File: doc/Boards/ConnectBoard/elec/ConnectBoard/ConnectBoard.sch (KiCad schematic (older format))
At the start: 20 parts

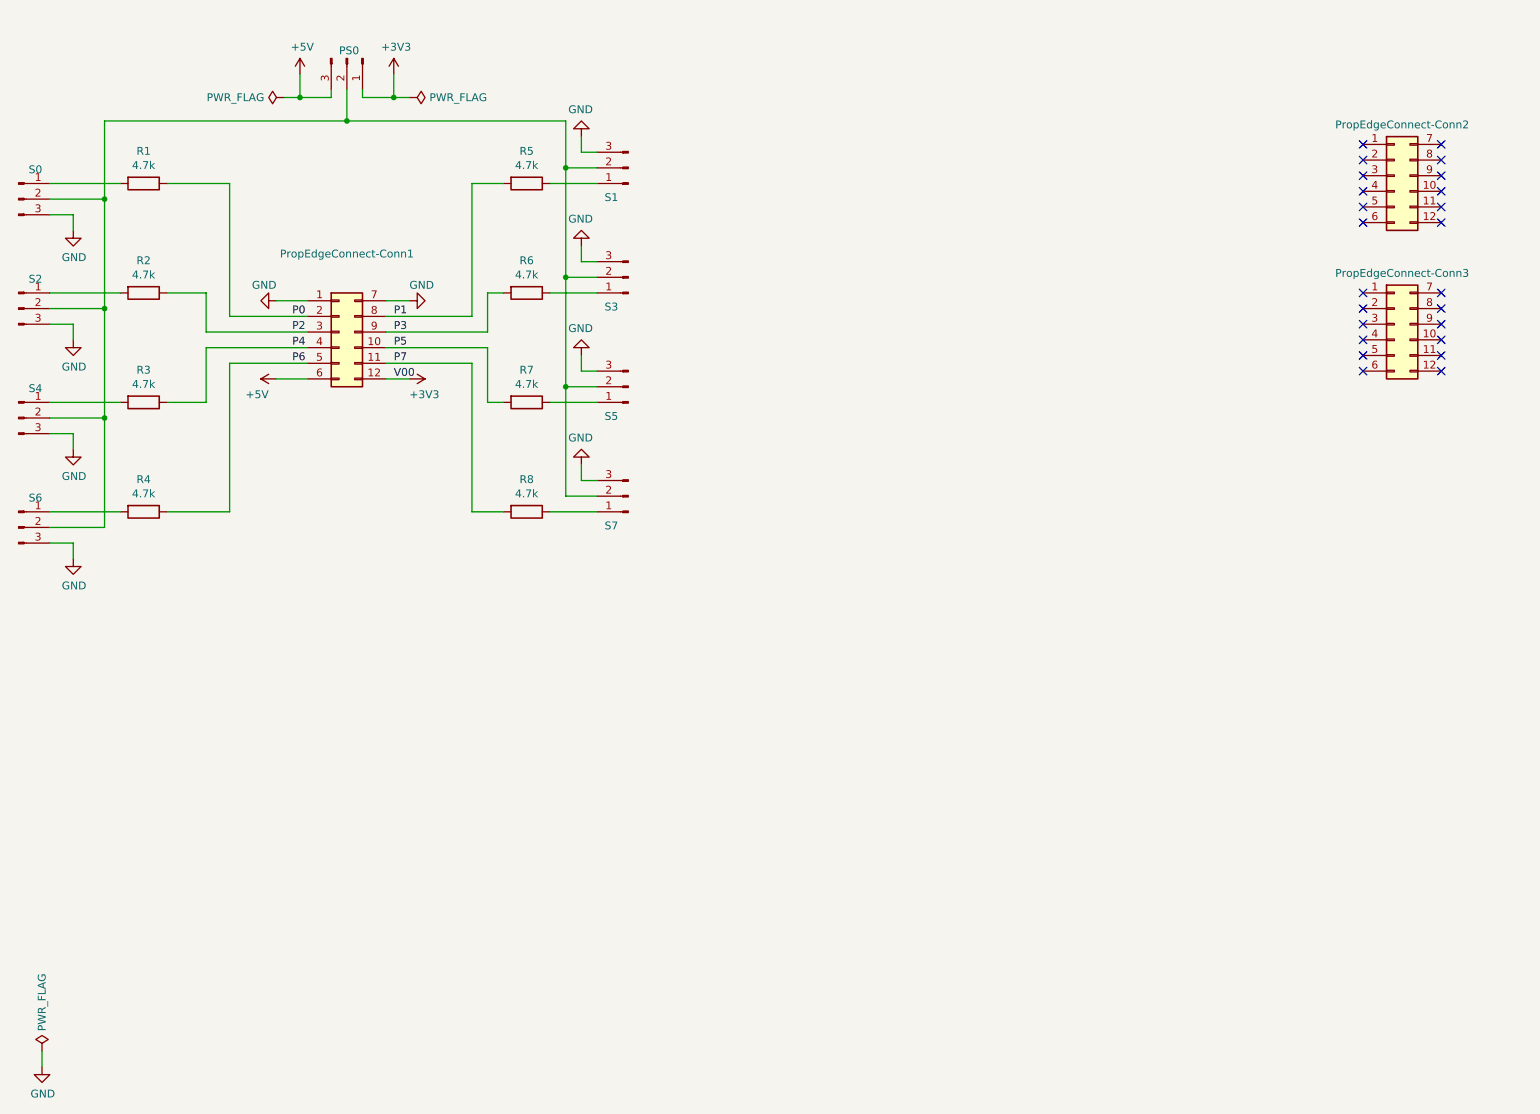
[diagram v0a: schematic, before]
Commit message: Updates
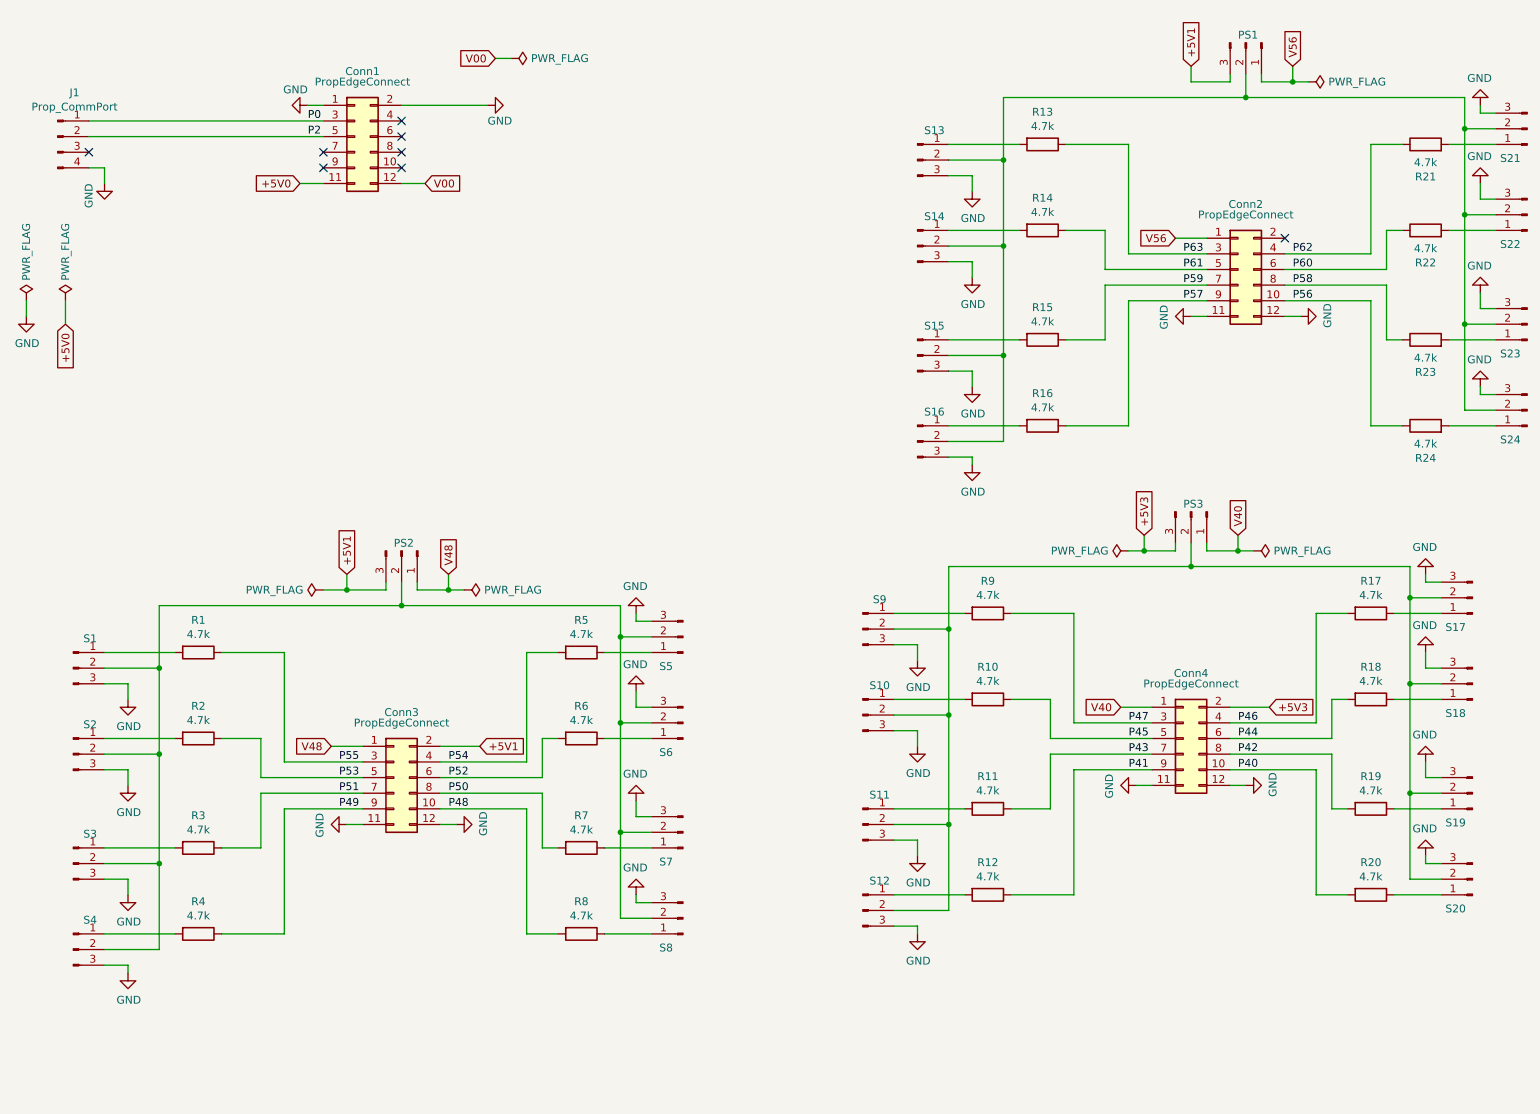
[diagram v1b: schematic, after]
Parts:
- removed PropEdgeConnect-Conn1: PropEdgeConnect-Conn1, Connector_PinSocket_2.54mm:PinSocket_2x06_P2.54mm_Vertical, symbol Connector_Generic:Conn_02x06_Top_Bottom
- removed PropEdgeConnect-Conn2: PropEdgeConnect-Conn2, Connector_PinSocket_2.54mm:PinSocket_2x06_P2.54mm_Vertical, symbol Connector_Generic:Conn_02x06_Top_Bottom
- removed PropEdgeConnect-Conn3: PropEdgeConnect-Conn3, Connector_PinSocket_2.54mm:PinSocket_2x06_P2.54mm_Vertical, symbol Connector_Generic:Conn_02x06_Top_Bottom
- added Conn1, Conn2, Conn3, Conn4: PropEdgeConnect, Connector_PinSocket_2.54mm:PinSocket_2x06_P2.54mm_Vertical, symbol Connector_Generic:Conn_02x06_Odd_Even
- added J1: Prop_CommPort, Connector_PinSocket_2.54mm:PinSocket_1x04_P2.54mm_Vertical, symbol Connector:Conn_01x04_Male
- added PS2, PS3: PowerSelect, Connector_PinHeader_2.54mm:PinHeader_1x03_P2.54mm_Vertical, symbol Connector:Conn_01x03_Male
- added R1, R10, R11, R12, R17, R18, R19, R2, R20, R3, R4, R5, R6, R7, R8, R9: 4.7k, Resistor_THT:R_Axial_DIN0207_L6.3mm_D2.5mm_P7.62mm_Horizontal, symbol Device:R
- added S1, S10, S11, S12, S17, S18, S19, S2, S20, S3, S4, S5, S6, S7, S8, S9: SonarConnect, Connector_PinHeader_2.54mm:PinHeader_1x03_P2.54mm_Vertical, symbol Connector:Conn_01x03_Male
- renumbered PS0 to PS1, R1 to R13, R2 to R14, R3 to R15, R4 to R16, R5 to R21, R6 to R22, R7 to R23, R8 to R24, S0 to S13, S2 to S14, S4 to S15, S6 to S16, S1 to S21, S3 to S22, S5 to S23, S7 to S24
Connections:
- net P1 is gone; now on an unnamed net: R21.2
- net P3 is gone; now on an unnamed net: R22.2
- net P5 is gone; now on an unnamed net: R23.2
- net P7 is gone; now on an unnamed net: R24.2
- net GND: now also Conn1.1 (Pin_1), Conn1.2 (Pin_2), Conn2.11 (Pin_11), Conn2.12 (Pin_12), Conn3.11 (Pin_11), Conn3.12 (Pin_12), Conn4.11 (Pin_11), Conn4.12 (Pin_12), J1.4 (Pin_4), S1.3 (Pin_3), S10.3 (Pin_3), S11.3 (Pin_3), S12.3 (Pin_3), S17.3 (Pin_3), S18.3 (Pin_3), S19.3 (Pin_3), S2.3 (Pin_3), S20.3 (Pin_3), S3.3 (Pin_3), S4.3 (Pin_3), S5.3 (Pin_3), S6.3 (Pin_3), S7.3 (Pin_3), S8.3 (Pin_3), S9.3 (Pin_3)
- net P0: now also Conn1.3 (Pin_3), J1.1 (Pin_1); no longer R13.1
- net P2: now also Conn1.5 (Pin_5), J1.2 (Pin_2); no longer R14.1
- net at S21.1 (Pin_1): no longer R21.1
- net at S22.1 (Pin_1): no longer R22.1
- net at S23.1 (Pin_1): no longer R23.1
- net at S24.1 (Pin_1): no longer R24.1
- net +3V3 renamed V56
- net V56: now also Conn2.1 (Pin_1)
- net +5V renamed +5V1
- net +5V1: now also Conn3.2 (Pin_2), PS2.3 (Pin_3)
- net P4 renamed P59
- net P59: now also Conn2.7 (Pin_7)
- net P6 renamed P57
- net P57: now also Conn2.9 (Pin_9)
- new net: R1.2, S1.1 (Pin_1)
- new net: PS2.2 (Pin_2), S1.2 (Pin_2), S2.2 (Pin_2), S3.2 (Pin_2), S4.2 (Pin_2), S5.2 (Pin_2), S6.2 (Pin_2), S7.2 (Pin_2), S8.2 (Pin_2)
- new net: R2.2, S2.1 (Pin_1)
- new net: R3.2, S3.1 (Pin_1)
- new net: R4.2, S4.1 (Pin_1)
- new net: R5.1, S5.1 (Pin_1)
- new net: R6.1, S6.1 (Pin_1)
- new net: R7.1, S7.1 (Pin_1)
- new net: R8.1, S8.1 (Pin_1)
- new net: R9.2, S9.1 (Pin_1)
- new net: PS3.2 (Pin_2), S10.2 (Pin_2), S11.2 (Pin_2), S12.2 (Pin_2), S17.2 (Pin_2), S18.2 (Pin_2), S19.2 (Pin_2), S20.2 (Pin_2), S9.2 (Pin_2)
- new net: R10.2, S10.1 (Pin_1)
- new net: R11.2, S11.1 (Pin_1)
- new net: R12.2, S12.1 (Pin_1)
- new net: R17.1, S17.1 (Pin_1)
- new net: R18.1, S18.1 (Pin_1)
- new net: R19.1, S19.1 (Pin_1)
- new net: R20.1, S20.1 (Pin_1)
- new net +5V0: Conn1.11 (Pin_11)
- new net +5V3: Conn4.2 (Pin_2), PS3.3 (Pin_3)
- new net P40: Conn4.10 (Pin_10), R20.2
- new net P41: Conn4.9 (Pin_9), R12.1
- new net P42: Conn4.8 (Pin_8), R19.2
- new net P43: Conn4.7 (Pin_7), R11.1
- new net P44: Conn4.6 (Pin_6), R18.2
- new net P45: Conn4.5 (Pin_5), R10.1
- new net P46: Conn4.4 (Pin_4), R17.2
- new net P47: Conn4.3 (Pin_3), R9.1
- new net P48: Conn3.10 (Pin_10), R8.2
- new net P49: Conn3.9 (Pin_9), R4.1
- new net P50: Conn3.8 (Pin_8), R7.2
- new net P51: Conn3.7 (Pin_7), R3.1
- new net P52: Conn3.6 (Pin_6), R6.2
- new net P53: Conn3.5 (Pin_5), R2.1
- new net P54: Conn3.4 (Pin_4), R5.2
- new net P55: Conn3.3 (Pin_3), R1.1
- new net P56: Conn2.10 (Pin_10), R24.1
- new net P58: Conn2.8 (Pin_8), R23.1
- new net P60: Conn2.6 (Pin_6), R22.1
- new net P61: Conn2.5 (Pin_5), R14.1
- new net P62: Conn2.4 (Pin_4), R21.1
- new net P63: Conn2.3 (Pin_3), R13.1
- new net V00: Conn1.12 (Pin_12)
- new net V40: Conn4.1 (Pin_1), PS3.1 (Pin_1)
- new net V48: Conn3.1 (Pin_1), PS2.1 (Pin_1)
- no-connect marks 24 -> 8
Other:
- moved on the sheet: PS1, R13, R14, R15, R16, R21, R22, R23, R24, S13, S14, S15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
